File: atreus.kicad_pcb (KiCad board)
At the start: 2 copper layers, 232 x 90 mm, 85 parts

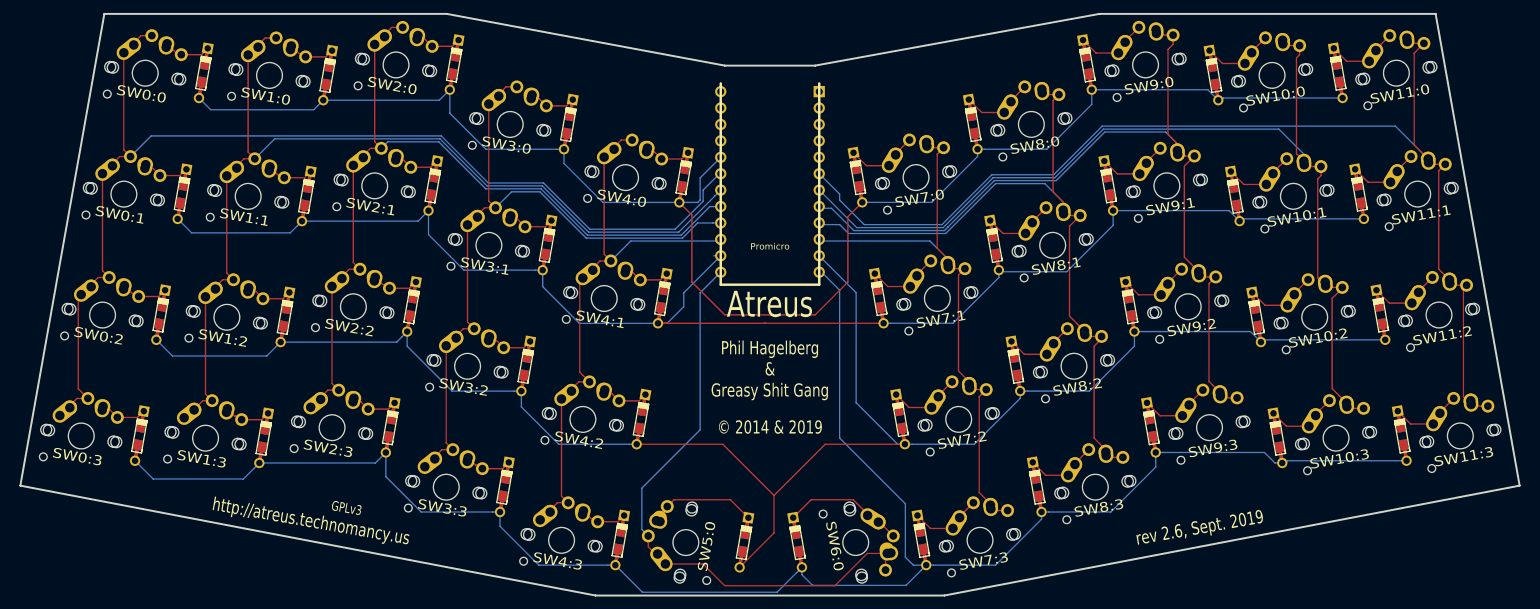
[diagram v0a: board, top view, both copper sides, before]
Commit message: new branch, only chocs.
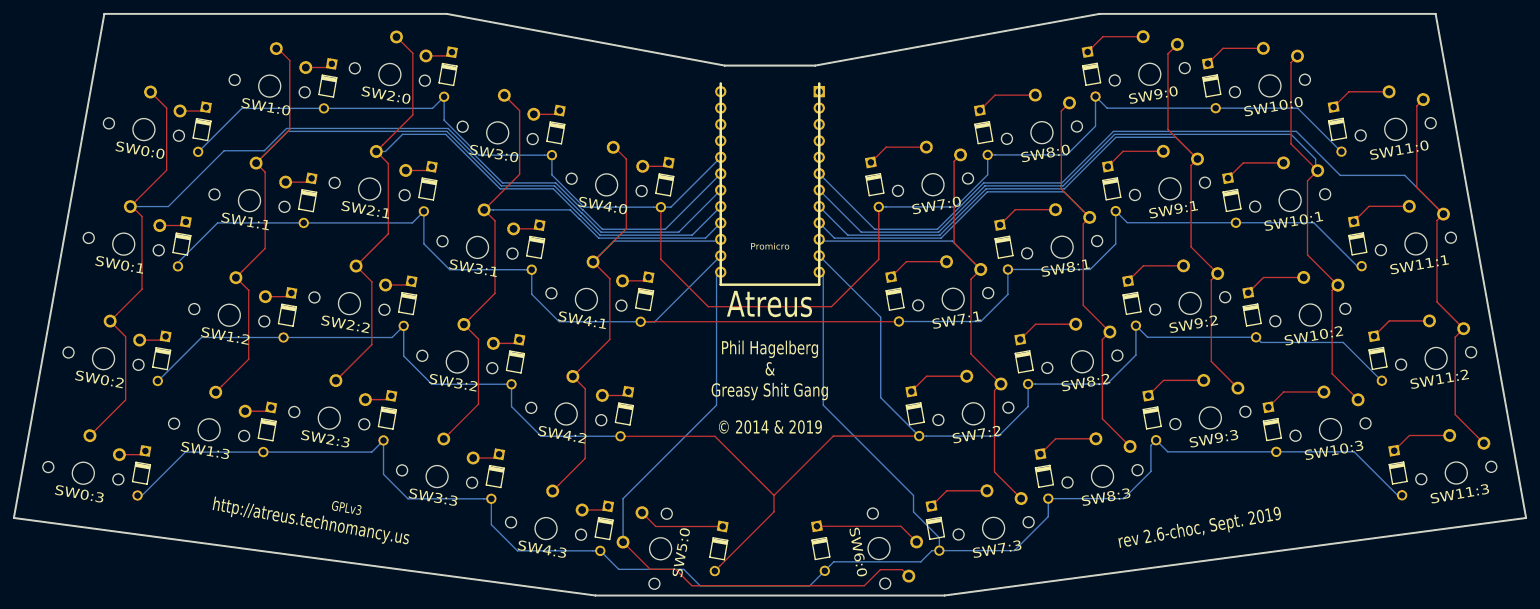
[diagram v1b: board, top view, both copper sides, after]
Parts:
- moved D0:0 8.72 mm to (46.1, 39.9)
- moved SW0:0 8.72 mm to (37.1, 39.9)
- moved D11:0 8.69 mm to (221.8, 39.9)
- moved SW11:0 8.69 mm to (230.8, 39.9)
- moved D0:1 7.74 mm to (43.0, 57.6)
- moved SW0:1 7.74 mm to (34.0, 57.6)
- moved D11:1 7.71 mm to (224.9, 57.6)
- moved SW11:1 7.71 mm to (233.9, 57.6)
- moved D0:2 6.75 mm to (39.9, 75.4)
- moved SW0:2 6.75 mm to (30.9, 75.4)
- moved D11:2 6.74 mm to (228.1, 75.3)
- moved SW11:2 6.74 mm to (237.1, 75.3)
- moved SW0:3 5.77 mm to (27.7, 93.1)
- moved D0:3 5.77 mm to (36.7, 93.1)
- moved D11:3 5.77 mm to (231.2, 93.0)
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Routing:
- net N-row-2: track 268.0 -> 277.5 mm
- net N-col-3: track 111.0 -> 101.7 mm
- net N-col-1: track 153.3 -> 144.6 mm
- net N-col-2: track 132.9 -> 125.4 mm
- net N-col-4: track 90.0 -> 83.6 mm
- net N-col-7: track 113.5 -> 107.4 mm
- net N-col-0: track 174.6 -> 168.9 mm
- net N-row-1: track 225.7 -> 231.2 mm
- net N-col-8: track 133.1 -> 128.0 mm
- net N-col-9: track 153.6 -> 148.9 mm
- net N-col-5: track 92.2 -> 96.5 mm
- net N-col-10: track 175.6 -> 171.5 mm
- net N-row-0: track 237.4 -> 241.2 mm
- net N-diode-20: track 17.0 -> 13.4 mm
- net N-diode-2: track 7.39 -> 4.26 mm
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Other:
- board size 232 x 90 mm -> 234 x 90 mm
- board text added: "rev 2.6-choc, Sept. 2019"
- board text removed: "rev 2.6, Sept. 2019"

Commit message: case for choc.
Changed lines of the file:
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@@
    (net 2 N-row-1)))
 (module Keebio-Parts:MX-Alps-Choc-1U-NoLED (layer Front)
-  (at 30.87048249320629 75.35086260162737 -10)
+  (at 30.8704824932063 75.35086260162736 -10)
   (fp_text
    reference
@@
    (net 5 N-col-0)))
 (module DIODE (layer Front)
-  (at 39.87048249320629 75.35086260162737 80)
+  (at 39.870482493206296 75.35086260162736 80)
   (attr smd)
   (fp_text
@@
    (net 2 N-row-1)))
 (module Keebio-Parts:MX-Alps-Choc-1U-NoLED (layer Front)
-  (at 50.333503824095345 68.62845226951004 -10)
+  (at 50.333503824095345 68.62845226951003 -10)
   (fp_text
    reference
@@
    (net 6 N-col-1)))
 (module DIODE (layer Front)
-  (at 59.333503824095345 68.62845226951004 80)
+  (at 59.333503824095345 68.62845226951003 80)
   (attr smd)
   (fp_text
@@
    (net 2 N-row-1)))
 (module Keebio-Parts:MX-Alps-Choc-1U-NoLED (layer Front)
-  (at 85.6129347548679 75.86459441853174 -10)
+  (at 85.61293475486791 75.86459441853172 -10)
   (fp_text
    reference
@@
    (net 8 N-col-3)))
 (module DIODE (layer Front)
-  (at 94.6129347548679 75.86459441853174 80)
+  (at 94.61293475486791 75.86459441853172 80)
   (attr smd)
   (fp_text
